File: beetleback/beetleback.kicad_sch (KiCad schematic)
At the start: 12 parts, among them J1 Conn_01x01_Male, J2 Conn_01x03_Male, J3 Conn_01x01_Male, U1 TA6586, U2 ATtiny412-SS, U3 ME6214A33M3G

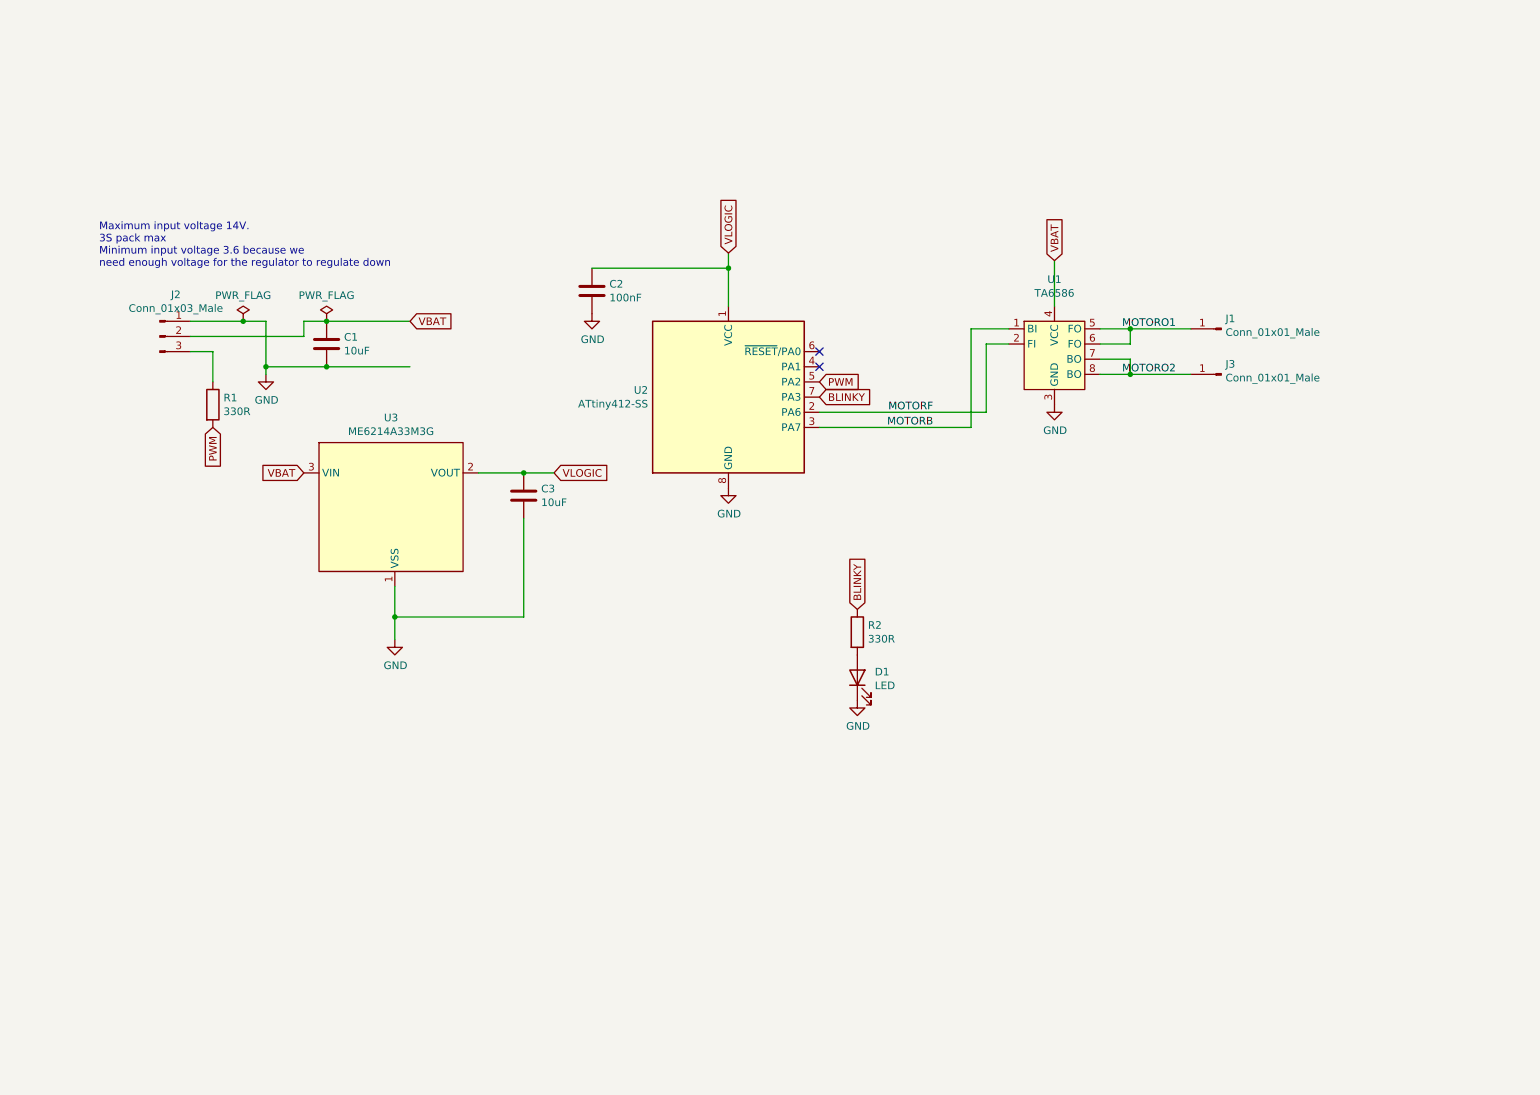
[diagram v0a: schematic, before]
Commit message: beetle motor esc back
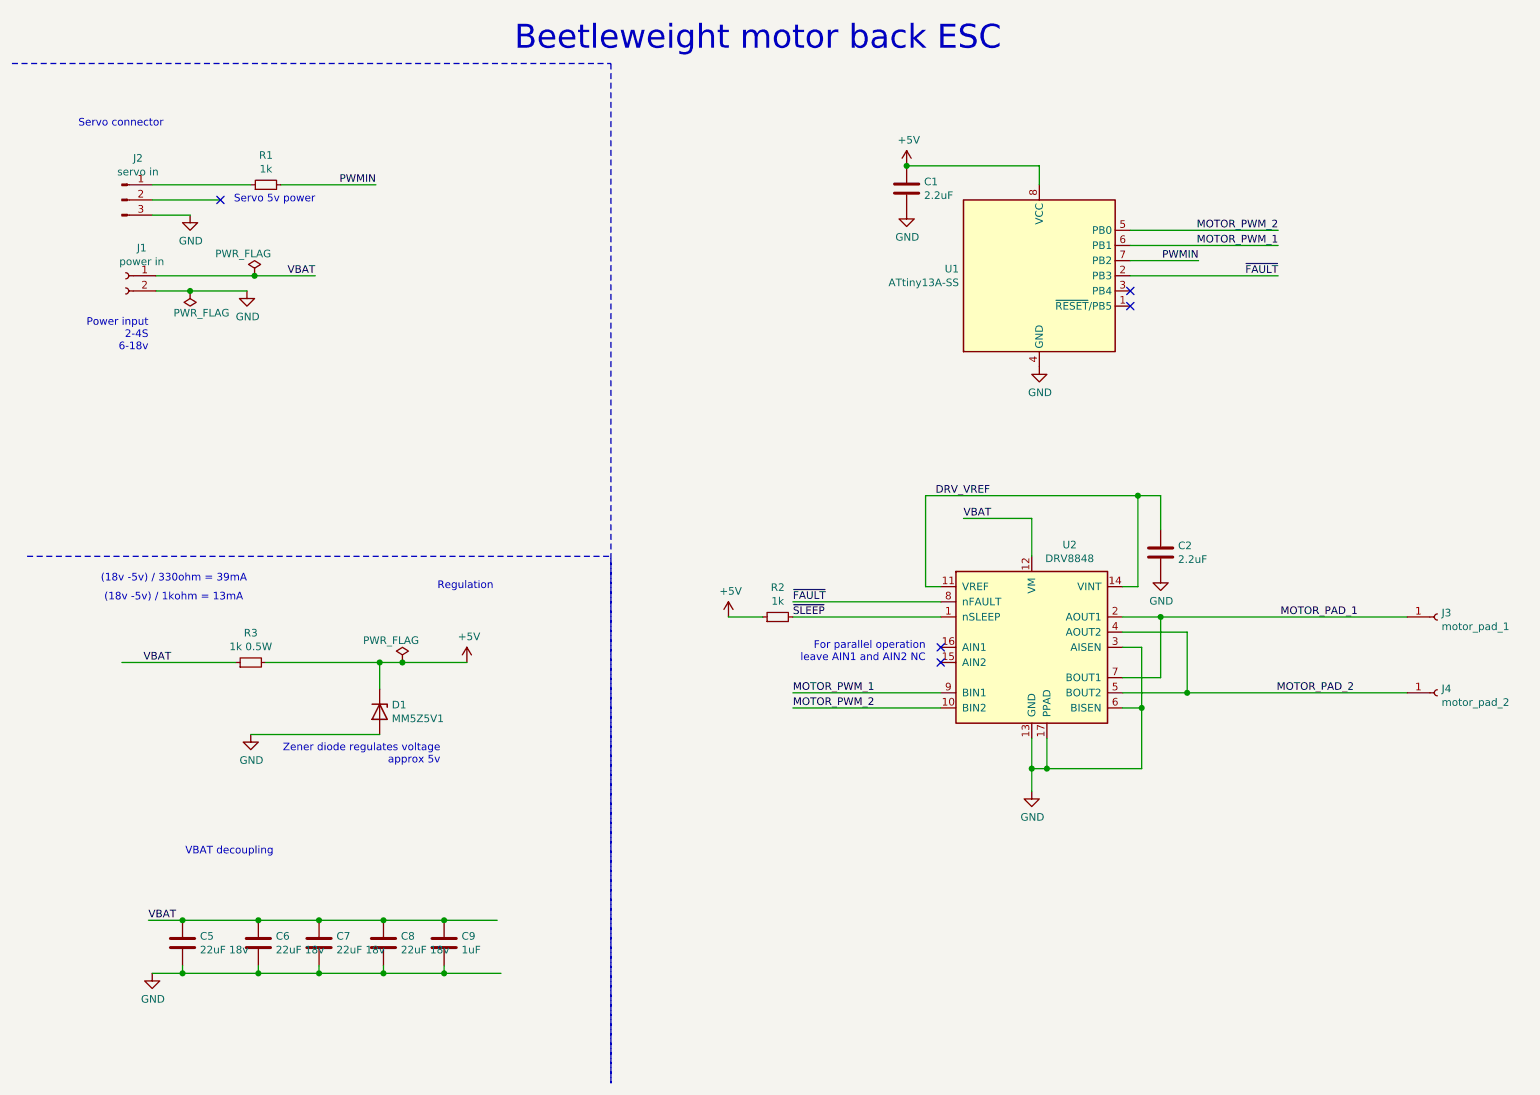
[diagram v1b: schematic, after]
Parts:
- removed C3: 10uF, Capacitor_SMD:C_0805_2012Metric, symbol Device:C
- removed D1: LED, LED_SMD:LED_0603_1608Metric_Castellated, symbol Device:LED
- removed J1, J3: Conn_01x01_Male, Connector_Wire:SolderWire-2sqmm_1x01_D2mm_OD3.9mm, symbol Connector:Conn_01x01_Male
- removed R1, R2: 330R, Resistor_SMD:R_0603_1608Metric, symbol Device:R
- removed U1: TA6586, Package_DIP:DIP-8_W7.62mm, symbol beetleback:TA6586
- removed U2: ATtiny412-SS, Package_SO:SOIC-8_3.9x4.9mm_P1.27mm, symbol MCU_Microchip_ATtiny:ATtiny412-SS
- removed U3: ME6214A33M3G, Package_TO_SOT_SMD:SOT-23, symbol beetleback:ME6214A33M3G
- added C5, C6, C7, C8: 22uF 18v, Capacitor_SMD:C_1206_3216Metric, symbol Device:C
- added C9: 1uF, Capacitor_SMD:C_0603_1608Metric, symbol Device:C
- added D1: MM5Z5V1, Diode_SMD:D_SOD-523, symbol Device:D_Zener
- added J1: power in, Connector_JST:JST_XA_B02B-XASK-1-A_1x02_P2.50mm_Vertical, symbol Connector:Conn_01x02_Female
- added J3: motor_pad_1, Connector_Pin:Pin_D1.3mm_L11.0mm, symbol Connector:Conn_01x01_Female
- added J4: motor_pad_2, Connector_Pin:Pin_D1.3mm_L11.0mm, symbol Connector:Conn_01x01_Female
- added R1, R2: 1k, Resistor_SMD:R_0603_1608Metric, symbol Device:R_Small
- added R3: 1k 0.5W, Capacitor_SMD:C_0805_2012Metric, symbol Device:R_Small
- added U1: ATtiny13A-SS, Package_SO:SOIC-8_3.9x4.9mm_P1.27mm, symbol MCU_Microchip_ATtiny:ATtiny13A-SS
- added U2: DRV8848, Package_SO:TSSOP-16-1EP_4.4x5mm_P0.65mm, symbol Driver_Motor:DRV8848
- C1: value 10uF -> 2.2uF; footprint Capacitor_SMD:C_0805_2012Metric -> Capacitor_SMD:C_0603_1608Metric; LCSC C15850 -> (none)
- C2: value 100nF -> 2.2uF; footprint Capacitor_SMD:C_0805_2012Metric -> Capacitor_SMD:C_0603_1608Metric; LCSC C49678 -> (none)
- J2: value Conn_01x03_Male -> servo in
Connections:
- net GND: now also J2.3 (Pin_3), C5.2, C6.2, C7.2, C8.2, C9.2, D1.2 (A), J1.2 (Pin_2), U1.4 (GND), U2.13 (GND), U2.17 (PPAD), U2.3 (AISEN), U2.6 (BISEN); no longer J2.1 (Pin_1)
- net VBAT: now also C5.1, C6.1, C7.1, C8.1, C9.1, J1.1 (Pin_1), R3.1, U2.12 (VM); no longer C1.1, J2.2 (Pin_2)
- net VLOGIC renamed DRV_VREF
- net DRV_VREF: now also U2.11 (VREF), U2.14 (VINT)
- new net: J2.1 (Pin_1), R1.1
- new net +5V: C1.1, D1.1 (K), R2.1, R3.2, U1.8 (VCC)
- new net MOTOR_PAD_1: J3.1 (Pin_1), U2.2 (AOUT1), U2.7 (BOUT1)
- new net MOTOR_PAD_2: J4.1 (Pin_1), U2.4 (AOUT2), U2.5 (BOUT2)
- new net MOTOR_PWM_1: U1.6 (PB1), U2.9 (BIN1)
- new net MOTOR_PWM_2: U1.5 (PB0), U2.10 (BIN2)
- new net PWMIN: R1.2, U1.7 (PB2)
- new net ~FAULT: U1.2 (PB3), U2.8 (nFAULT)
- new net ~SLEEP: R2.2, U2.1 (nSLEEP)
- no-connect marks 2 -> 5
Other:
- note added: "(18v -5v) / 1kohm = 13mA"
- note added: "(18v -5v) / 330ohm = 39mA"
- note added: "Beetleweight motor back ESC"
- note added: "For parallel operation leave AIN1 and AIN2 NC"
- note added: "Power input 2-4S 6-18v"
- note added: "Regulation"
- note added: "Servo 5v power"
- note added: "Servo connector"
- note added: "VBAT decoupling"
- note added: "Zener diode regulates voltage approx 5v"
- note removed: "Maximum input voltage 14V. 3S pack max Minimum input voltage 3.6 because we need enough voltage for the regulator to regulate down"
- moved on the sheet: J2
